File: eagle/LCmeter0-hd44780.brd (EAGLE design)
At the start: 64.8 x 50.8 mm, 26 parts, among them J1 22-27-2021-02, K1 DS2Y

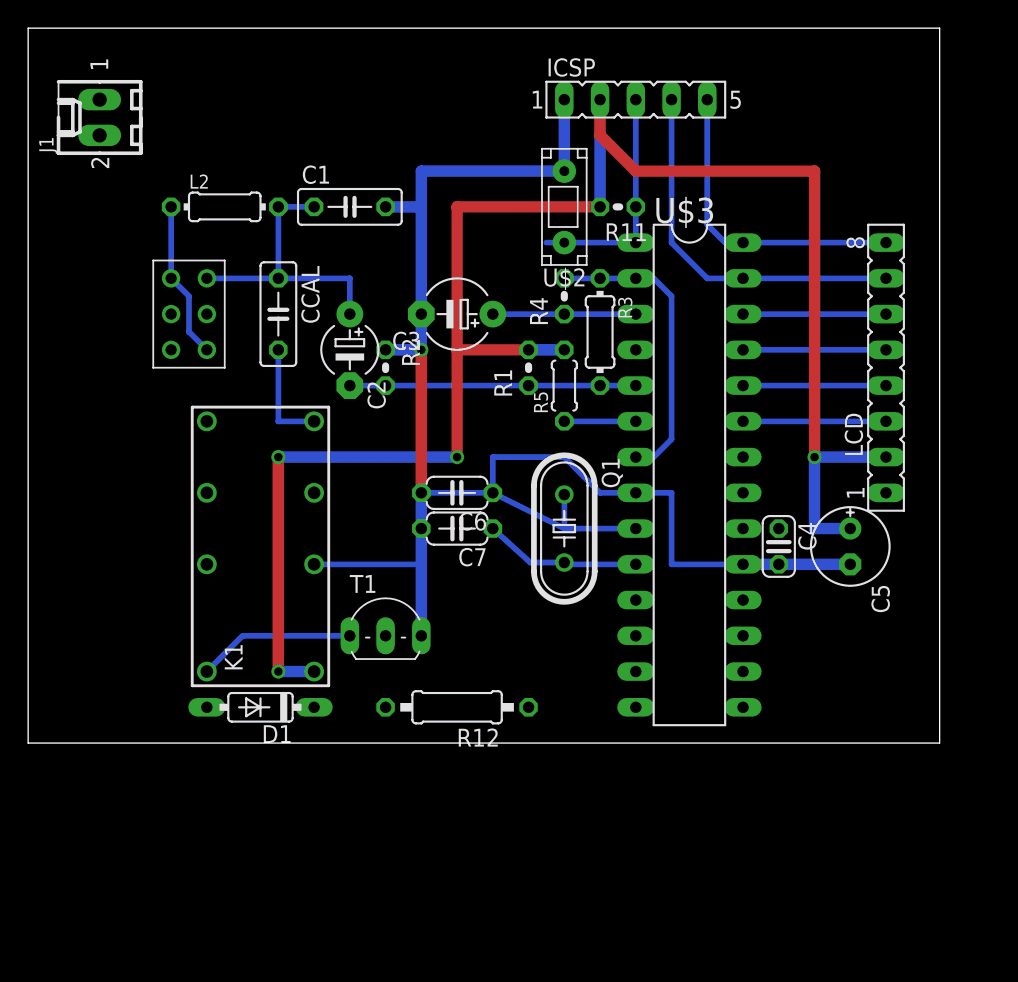
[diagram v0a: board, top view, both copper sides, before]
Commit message: ...
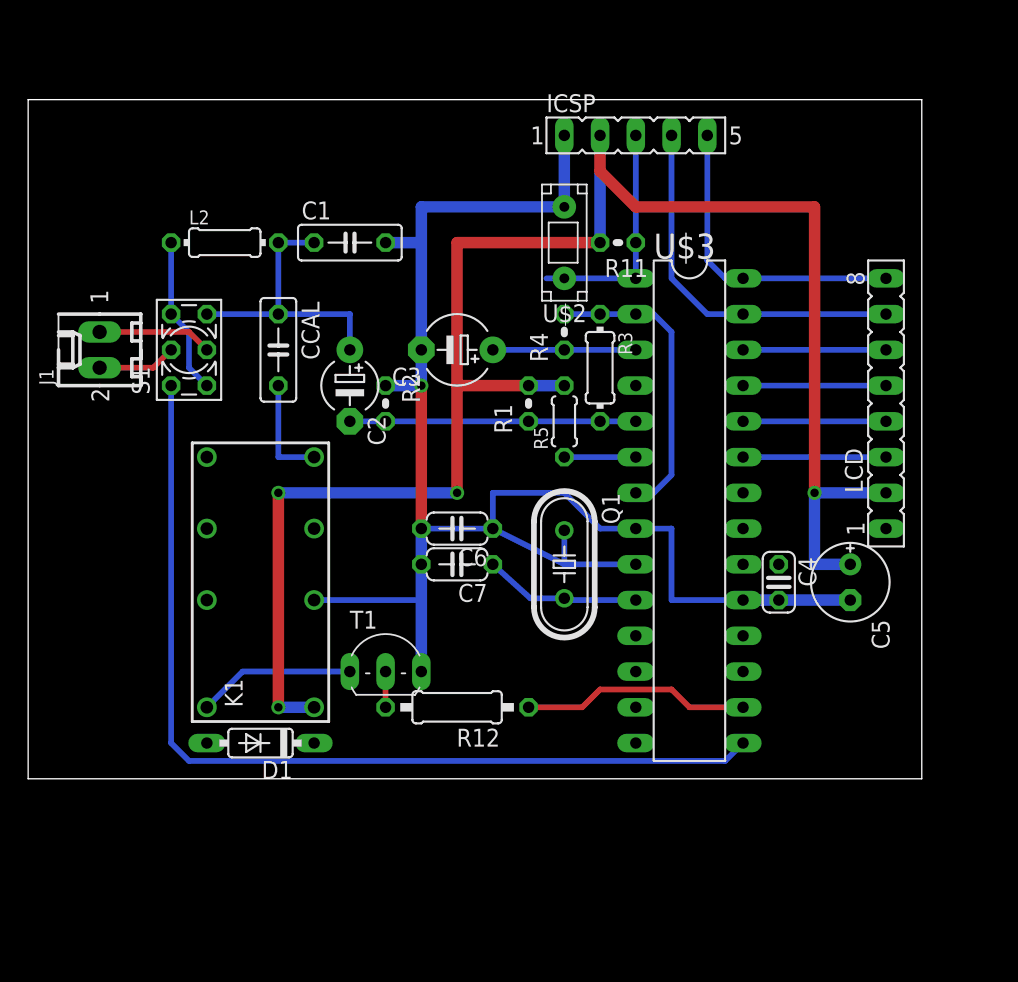
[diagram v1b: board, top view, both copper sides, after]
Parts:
- removed U$4: S-DPDT, lc-meter:DPDT
- added S1: 9450-2, switch-misc:9450-2
- moved J1 16.5 mm to (5.08, 30.5)
- moved U$2 2.54 mm to (39.4, 41.9)
- moved C3 2.54 mm to (30.5, 30.5)
- moved CCAL 2.54 mm to (17.8, 30.5)
- moved R5 2.54 mm to (38.1, 25.4)
- moved C4 2.54 mm to (53.3, 14.0)
- moved C5 2.54 mm to (58.4, 14.0)
- moved C7 2.54 mm to (30.5, 15.2)
- moved K1 2.54 mm to (16.5, 14.0)
- moved Q1 2.54 mm to (38.1, 15.2)
- moved D1 2.54 mm to (16.5, 2.54)
- moved T1 2.54 mm to (25.4, 7.62)
- moved C1 2.54 mm to (22.9, 38.1)
- moved C2 2.54 mm to (22.9, 27.9)
- moved C6 2.54 mm to (30.5, 17.8)
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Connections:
- net L/C: now also S1.4; no longer U$4.2-3
- net N$23: now also S1.3; no longer U$4.1-2
- net N$24: now also S1.1, S1.6; no longer U$4.1-3, U$4.2-2
- net N$5: now also S1.2; no longer U$4.1-1
- net N$8: now also S1.5; no longer U$4.2-1
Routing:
- net L/C: track 0.00 -> 67.1 mm
- net RELAY: track 0.00 -> 16.3 mm
- net N$5: track 0.00 -> 8.15 mm
- net N$8: track 0.00 -> 5.61 mm
- net N$19: track 0.00 -> 2.54 mm
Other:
- board size 64.8 x 50.8 mm -> 63.5 x 48.3 mm

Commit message: ...
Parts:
- U$2: device lc-meter:PB-5-1 -> mcu:PB-5-1
- U$3: device lc-meter:DIL28-3 -> mcu:DIL28-3
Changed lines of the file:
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@@
 <attribute name="OC_FARNELL" value="unknown" x="60.96" y="26.67" size="1.778" layer="27" rot="R90" display="off"/>
 </element>
-<element name="U$3" library="lc-meter" package="DIL28-3" value="PIC16F876A-X/SP-COMP-B" x="46.99" y="19.05" rot="R270"/>
+<element name="U$3" library="mcu" package="DIL28-3" value="PIC16F876A-X/SP-COMP-B" x="46.99" y="19.05" rot="R270"/>
 <element name="ICSP" library="con-lsta" package="FE05-1" value="" x="43.18" y="45.72">
 <attribute name="MPN" value="" x="43.18" y="45.72" size="1.778" layer="27" display="off"/>
@@
 <element name="C4" library="resistor" package="C025-024X044" value="" x="53.34" y="13.97" rot="R270"/>
 <element name="C5" library="rcl" package="E2,5-6E" value="" x="58.42" y="13.97" rot="R270"/>
-<element name="U$2" library="lc-meter" package="PB-5-1" value="PB-5-2" x="39.37" y="41.91" rot="R180"/>
+<element name="U$2" library="mcu" package="PB-5-1" value="PB-5-2" x="39.37" y="41.91" rot="R180"/>
 <element name="J1" library="con-molex" package="6410-02" value="22-27-2021-02" x="5.08" y="30.48" rot="R90">
 <attribute name="MPN" value="" x="5.08" y="30.48" size="1.778" layer="27" rot="R90" display="off"/>

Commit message: ...
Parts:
- C4: device resistor:C025-024X044 -> r:C025-024X044
- D1: device diode:DO35-7 -> d:DO35-7
- Q1: device crystal:HC49/S -> q:HC49/S
- T1: device transistor:TO92-CBE -> t:TO92-CBE
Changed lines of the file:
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@@
 <element name="C7" library="rcl" package="C050-024X044" value="22pF" x="30.48" y="15.24" rot="R180"/>
 <element name="CCAL" library="rcl" package="C050-025X075" value="1nF" x="17.78" y="30.48" rot="R270"/>
-<element name="D1" library="diode" package="DO35-7" value="1N4148" x="16.51" y="2.54" rot="R180"/>
+<element name="D1" library="d" package="DO35-7" value="1N4148" x="16.51" y="2.54" rot="R180"/>
 <element name="K1" library="relay" package="DS2Y" value="DS2Y" x="16.51" y="13.97" rot="R90">
 <attribute name="OC_FARNELL" value="unknown" x="16.51" y="13.97" size="1.778" layer="27" rot="R90" display="off"/>
@@
 </element>
 <element name="L2" library="rcl" package="0204/7" value="100uH" x="13.97" y="38.1"/>
-<element name="Q1" library="crystal" package="HC49/S" value="" x="38.1" y="15.24" rot="R270">
+<element name="Q1" library="q" package="HC49/S" value="" x="38.1" y="15.24" rot="R270">
 <attribute name="OC_FARNELL" value="1667008" x="38.1" y="15.24" size="1.778" layer="27" rot="R270" display="off"/>
 <attribute name="OC_NEWARK" value="unknown" x="38.1" y="15.24" size="1.778" layer="27" rot="R270" display="off"/>
@@
 <element name="R4" library="rcl" package="0204V" value="47k" x="38.1" y="31.75" rot="R90"/>
 <element name="R5" library="rcl" package="0204/5" value="4.7k" x="38.1" y="25.4" rot="R90"/>
-<element name="T1" library="transistor" package="TO92-CBE" value="" x="25.4" y="7.62"/>
+<element name="T1" library="t" package="TO92-CBE" value="" x="25.4" y="7.62"/>
 <element name="LCD" library="con-lsta" package="FE08" value="" x="60.96" y="26.67" rot="R90">
 <attribute name="MPN" value="" x="60.96" y="26.67" size="1.778" layer="27" rot="R90" display="off"/>
@@
 <attribute name="OC_FARNELL" value="unknown" x="43.18" y="45.72" size="1.778" layer="27" display="off"/>
 </element>
-<element name="C4" library="resistor" package="C025-024X044" value="" x="53.34" y="13.97" rot="R270"/>
+<element name="C4" library="r" package="C025-024X044" value="" x="53.34" y="13.97" rot="R270"/>
 <element name="C5" library="rcl" package="E2,5-6E" value="" x="58.42" y="13.97" rot="R270"/>
 <element name="U$2" library="mcu" package="PB-5-1" value="PB-5-2" x="39.37" y="41.91" rot="R180"/>
